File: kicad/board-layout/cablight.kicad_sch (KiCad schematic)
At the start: 16 parts, among them J1 Screw_Term_1x2_2.54mm, J2 Screw_Term_1x2_2.54mm, P1 Pololu D24V10F5, Q1 IRLB8721PBF, SW1 PEC11, SW3 switch_SPDT_SLW_121586

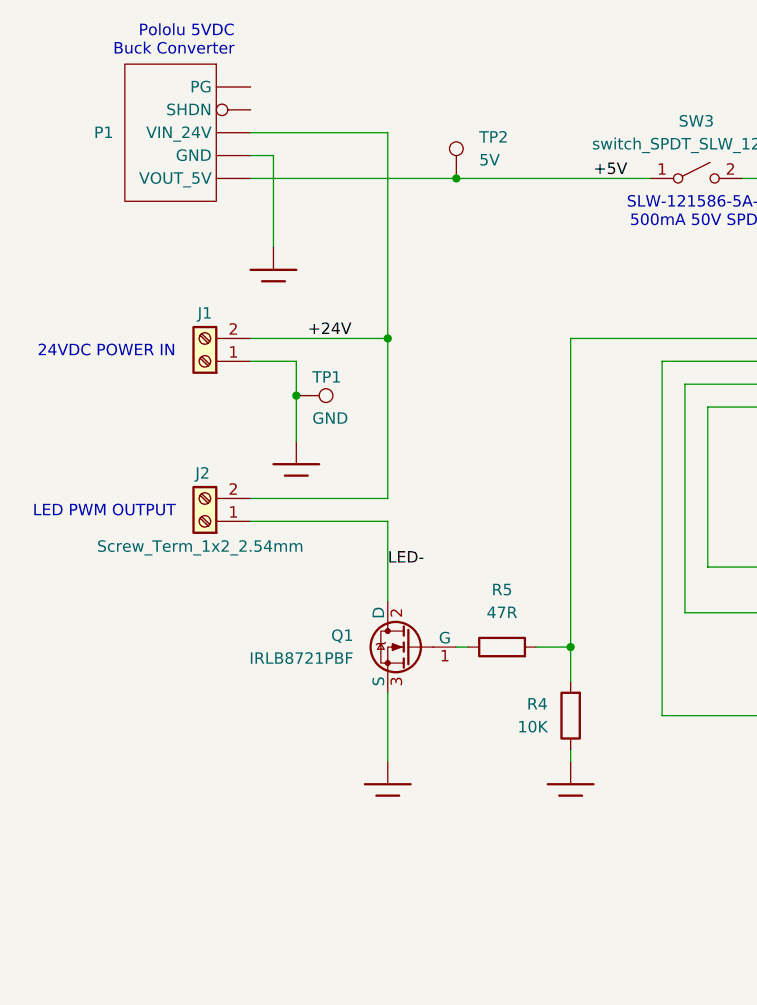
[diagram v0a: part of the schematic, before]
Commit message: board updates
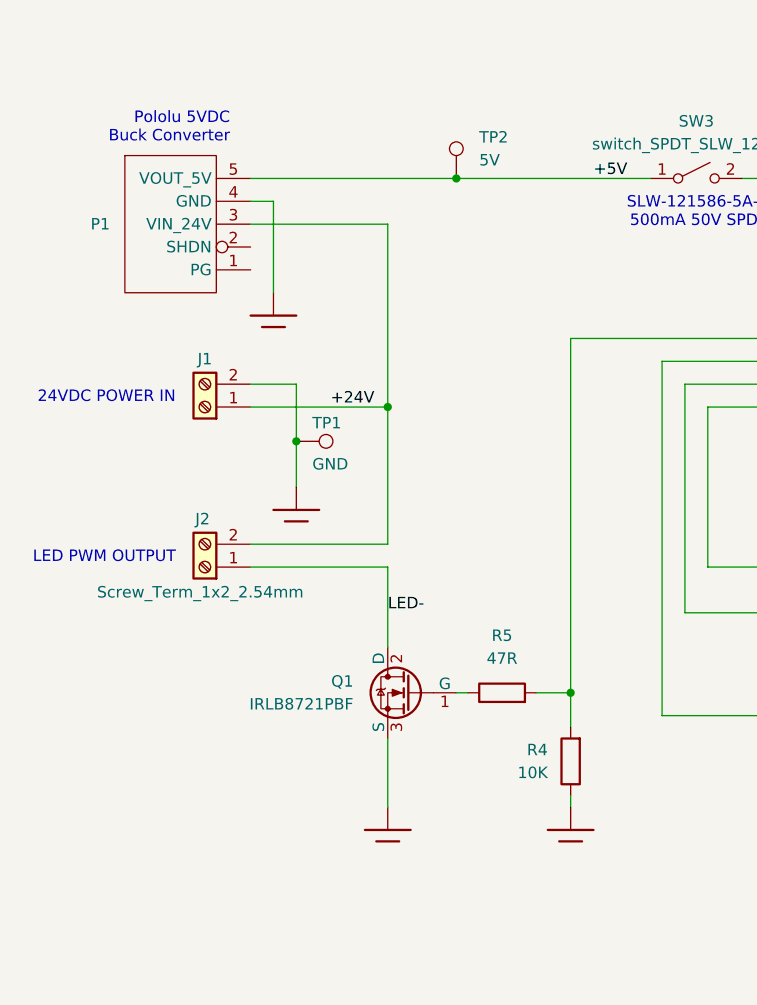
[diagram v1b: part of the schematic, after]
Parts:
- P1: symbol Power Supply Module:Pololu_0J8557_24V -> user:Pololu_0J8557_24V
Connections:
- net +24V: now also J1.1 (Pin_1), P1.3 (VIN_24V); no longer J1.2 (Pin_2), P1. (VOUT_5V)
- net +5V: now also P1.5 (VOUT_5V); no longer P1. (VOUT_5V)
- net at TP1.1: now also J1.2 (Pin_2); no longer J1.1 (Pin_1)
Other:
- moved on the sheet: J1, J2, Q1, R4, R5, TP1
